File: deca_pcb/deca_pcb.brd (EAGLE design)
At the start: 68.2 x 80 mm, 8 parts, among them IC1 DWM1000, IC2 LM340H-18, U1 ATMEGA328P-PU, X1 MINI-USB-32005-301, X2 332-06

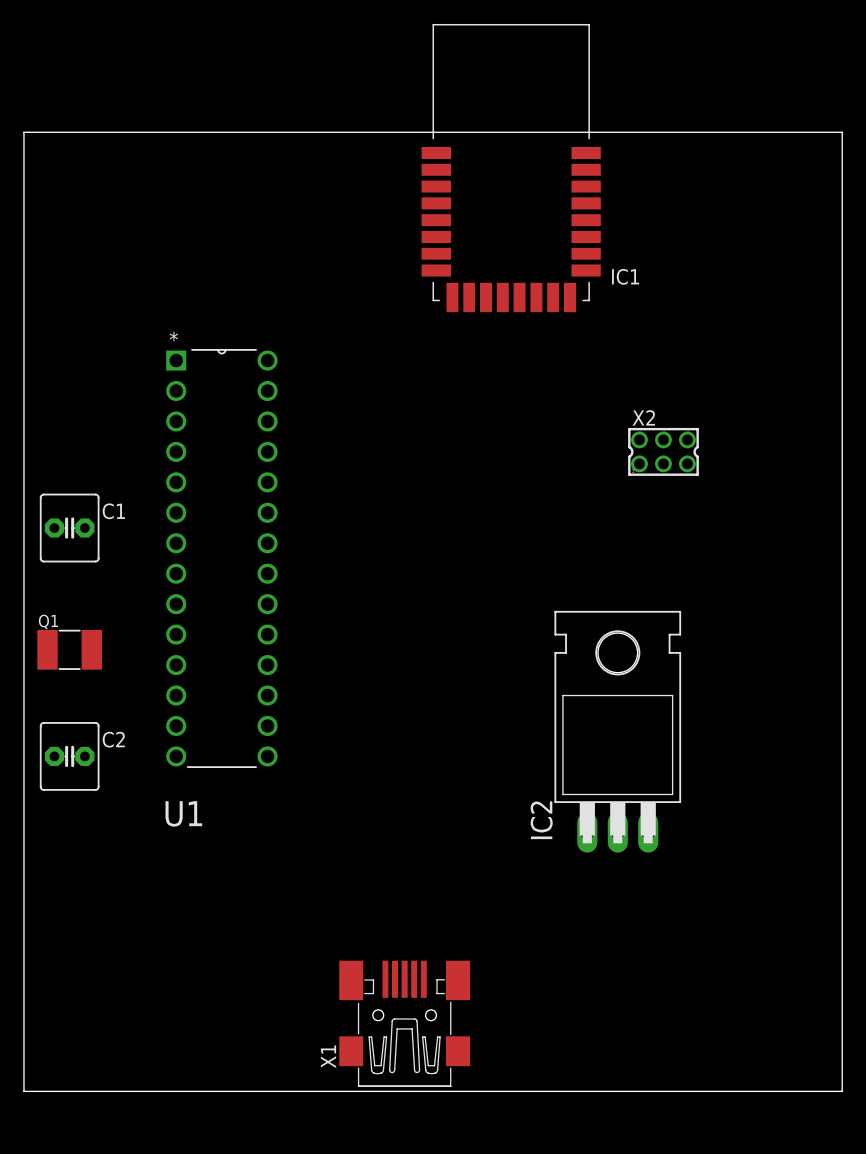
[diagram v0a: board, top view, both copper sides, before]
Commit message: board pcb done
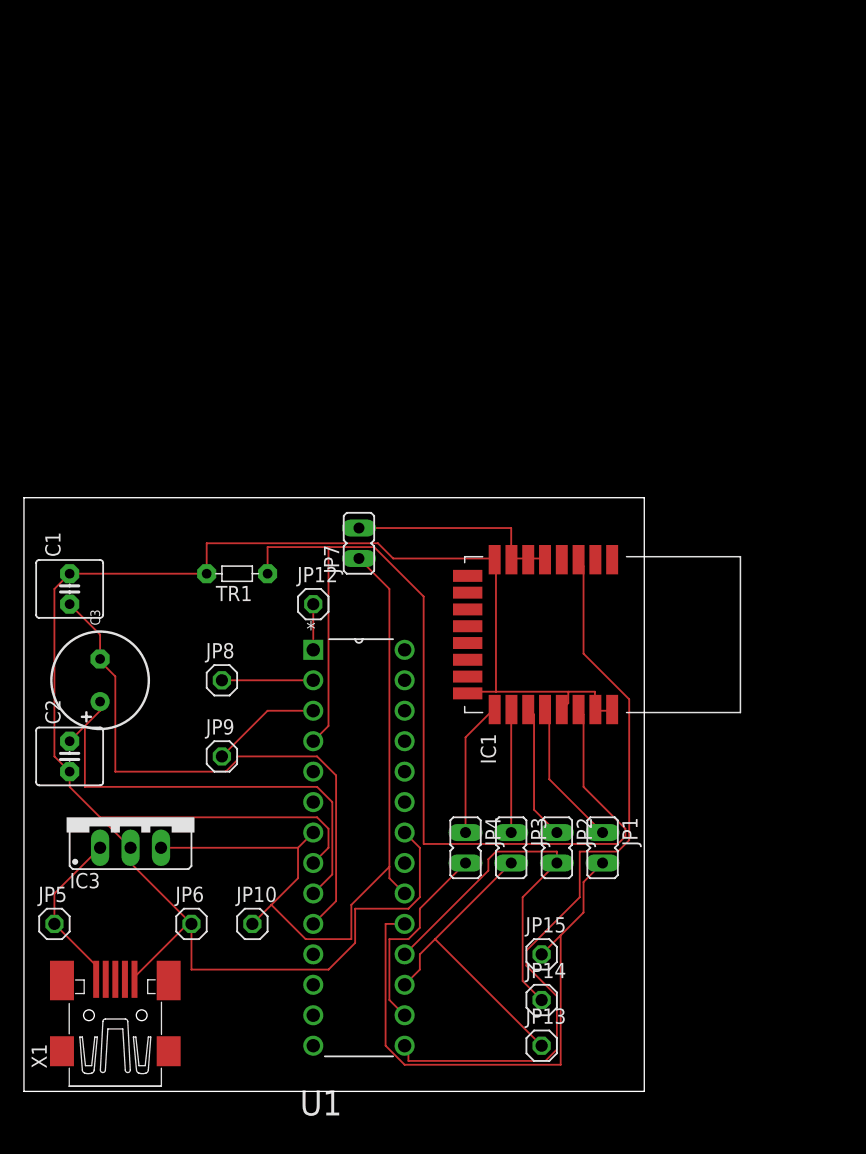
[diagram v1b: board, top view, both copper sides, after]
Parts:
- removed IC2: LM340H-18, linear:TO220H
- removed Q1: (no value), crystal-geyer_V1_0:5.0X3.2_2
- removed X2: 332-06, con-garry:332-06
- added C3: (no value), microbuilder:CELEC_3.5MM_8MM
- added IC3: (no value), lf33:TO220S
- added JP1, JP2, JP3, JP4, JP7: (no value), jumper:JP1
- added JP10, JP12, JP13, JP14, JP15, JP5, JP6, JP8, JP9: (no value), con-pinhead:1X01
- added TR1: (no value), discrete:R-5
- moved IC1 40.1 mm to (48.3, 38.1), turned to 270 degrees
- moved U1 26.7 mm to (31.8, 3.81)
- moved X1 24.1 mm to (7.62, 6.35)
- moved C1 5.08 mm to (3.81, 41.9), turned to 90 degrees
- turned C2 to 90 degrees
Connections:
- new net N$13: C1.2, C2.1, IC1.16, IC1.21, IC1.23, IC1.24, IC1.8, IC3.2, JP6.1, TR1.2, U1.22, U1.8, X1.5
- new net N$14: IC1.19, JP2.1
- new net N$15: IC1.18, JP3.1
- new net N$16: IC1.17, JP4.1
- new net N$17: JP8.1, U1.2
- new net N$18: JP9.1, U1.3
- new net N$19: JP12.1, U1.1
- net N$1: now also JP1.2, JP15.1; no longer IC1.20, X2.3
- net N$10: now also IC3.1, JP5.1; no longer IC2.1
- net N$11: now also IC1.20, JP1.1; no longer C1.2, C2.1, IC1.16, IC1.21, IC1.23, IC1.24, IC1.8, IC2.2, U1.22, U1.8, X1.5, X2.6
- net N$12: now also IC3.3, JP10.1, JP7.1; no longer IC1.5, IC1.6, IC1.7, IC2.3, X2.2
- net N$2: now also JP14.1, JP2.2; no longer IC1.19, X2.1
- net N$3: now also JP13.1, JP3.2; no longer IC1.18, X2.4
- net N$4: now also JP4.2; no longer IC1.17
- net N$5: now also TR1.1
- net N$7: now also C3.+; no longer Q1.2
- net N$8: now also C3.-; no longer Q1.1
- net N$9: now also IC1.5, IC1.6, IC1.7, JP7.2; no longer U1.1, X2.5
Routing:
- net N$13: track 0.00 -> 161.9 mm
- net N$5: track 0.00 -> 83.6 mm
- net N$12: track 0.00 -> 65.9 mm
- net N$6: track 0.00 -> 63.2 mm
- net N$8: track 0.00 -> 48.5 mm
- net N$1: track 0.00 -> 47.5 mm
- net N$7: track 0.00 -> 38.9 mm
- net N$2: track 0.00 -> 31.0 mm
- net N$3: track 0.00 -> 26.4 mm
- net N$9: track 0.00 -> 18.2 mm
- net N$4: track 0.00 -> 16.8 mm
- net N$10: track 0.00 -> 14.0 mm
- net N$11: track 0.00 -> 12.2 mm
- net N$16: track 0.00 -> 11.3 mm
- net N$14: track 0.00 -> 11.3 mm
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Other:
- board size 68.2 x 80 mm -> 51.7 x 49.5 mm
